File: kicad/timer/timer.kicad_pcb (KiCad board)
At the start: 4 copper layers, 71.1 x 58.4 mm, 18 parts, among them J1 Conn_01x01_Pin, J2 Conn_01x01_Pin, SW1 SW_Push, U1 ATmega328P-P, U2 L7805, Y1 Crystal

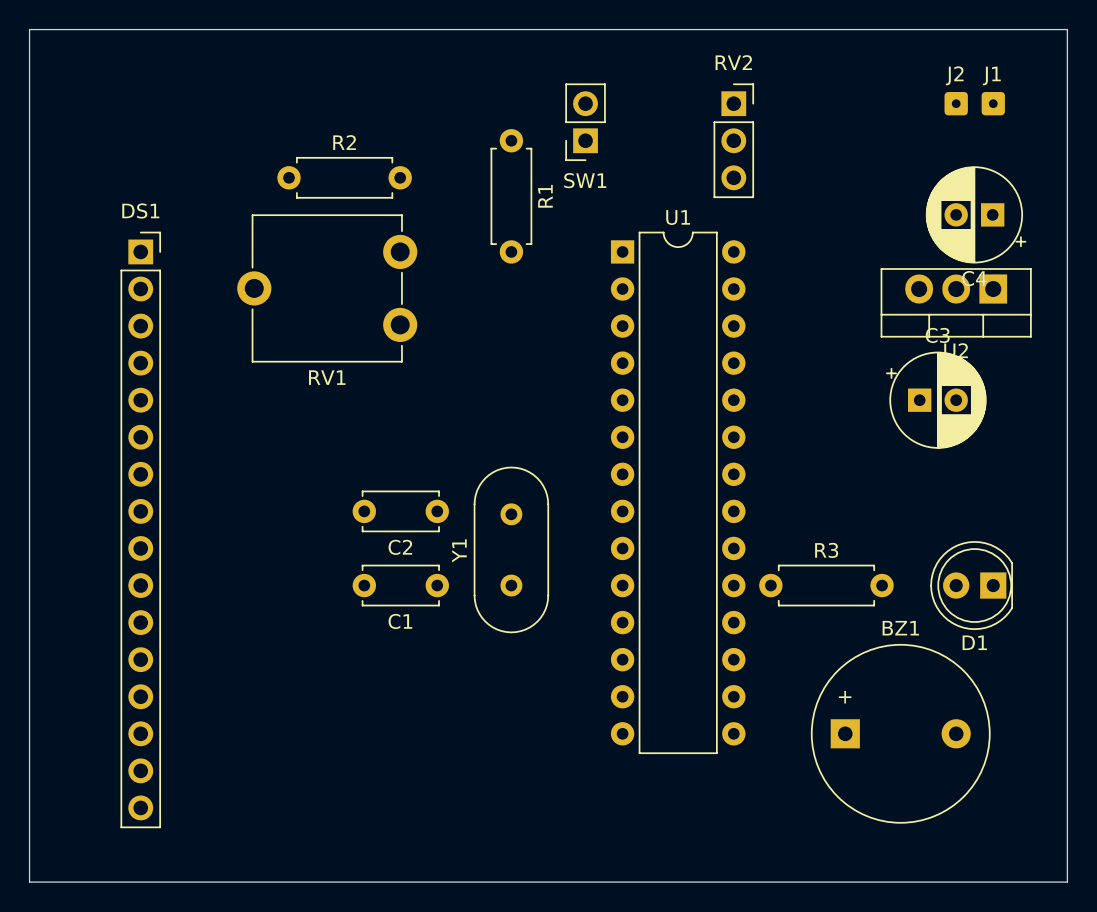
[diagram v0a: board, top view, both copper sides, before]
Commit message: Route wire tracks
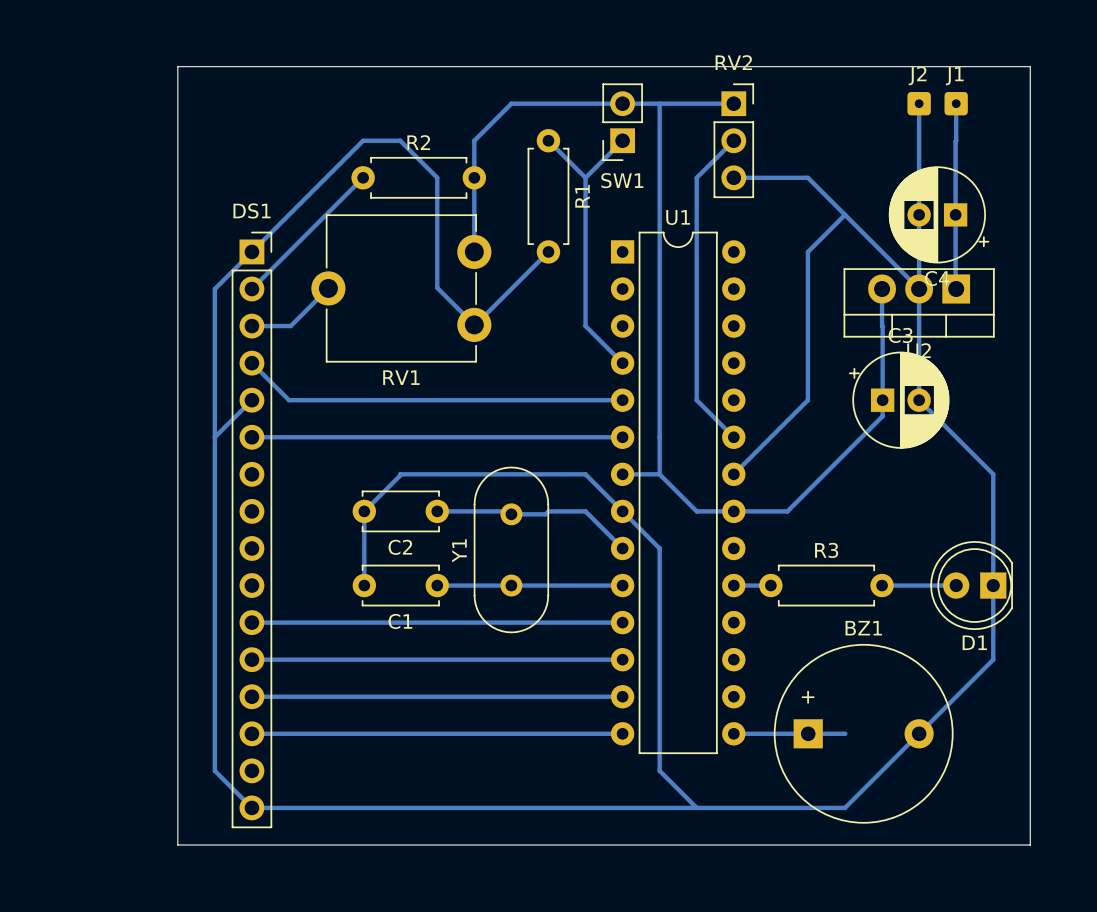
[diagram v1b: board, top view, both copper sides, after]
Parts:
- moved DS1 7.62 mm to (106.7, 83.8)
- moved R2 5.08 mm to (114.3, 78.7)
- moved RV1 5.08 mm to (121.9, 83.8)
- moved SW1 2.54 mm to (132.1, 76.2)
- moved R1 2.54 mm to (127.0, 76.2)
- moved BZ1 2.54 mm to (144.8, 116.8)
- moved C3 2.54 mm to (149.9, 94.0)
- moved C4 2.54 mm to (154.9, 81.3)
- moved J1 2.54 mm to (154.9, 73.7)
- moved J2 2.54 mm to (152.4, 73.7)
- moved U2 2.54 mm to (154.9, 86.4)
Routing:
- net GND: track 0.00 -> 258.3 mm
- net +5V: track 0.00 -> 82.2 mm
- net Net-(DS1-RS): track 0.00 -> 26.5 mm
- net Net-(DS1-E): track 0.00 -> 25.4 mm
- net Net-(DS1-D7): track 0.00 -> 25.4 mm
- net Net-(DS1-D6): track 0.00 -> 25.4 mm
- net Net-(DS1-D5): track 0.00 -> 25.4 mm
- net Net-(DS1-D4): track 0.00 -> 25.4 mm
- net Net-(U1-PC0): track 0.00 -> 22.4 mm
- net Net-(U1-PD2): track 0.00 -> 20.9 mm
- net Net-(U1-XTAL1/PB6): track 0.00 -> 13.9 mm
- net +9V: track 0.00 -> 12.7 mm
- net Net-(U1-XTAL2/PB7): track 0.00 -> 12.7 mm
- net Net-(DS1-VDD): track 0.00 -> 10.8 mm
- net Net-(BZ1-+): track 0.00 -> 7.64 mm
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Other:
- board size 71.1 x 58.4 mm -> 58.4 x 53.3 mm
